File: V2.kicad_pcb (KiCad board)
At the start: 2 copper layers, 54.1 x 26 mm, 13 parts, among them SW1 SW_SPST, U1 CH32V003JxMx

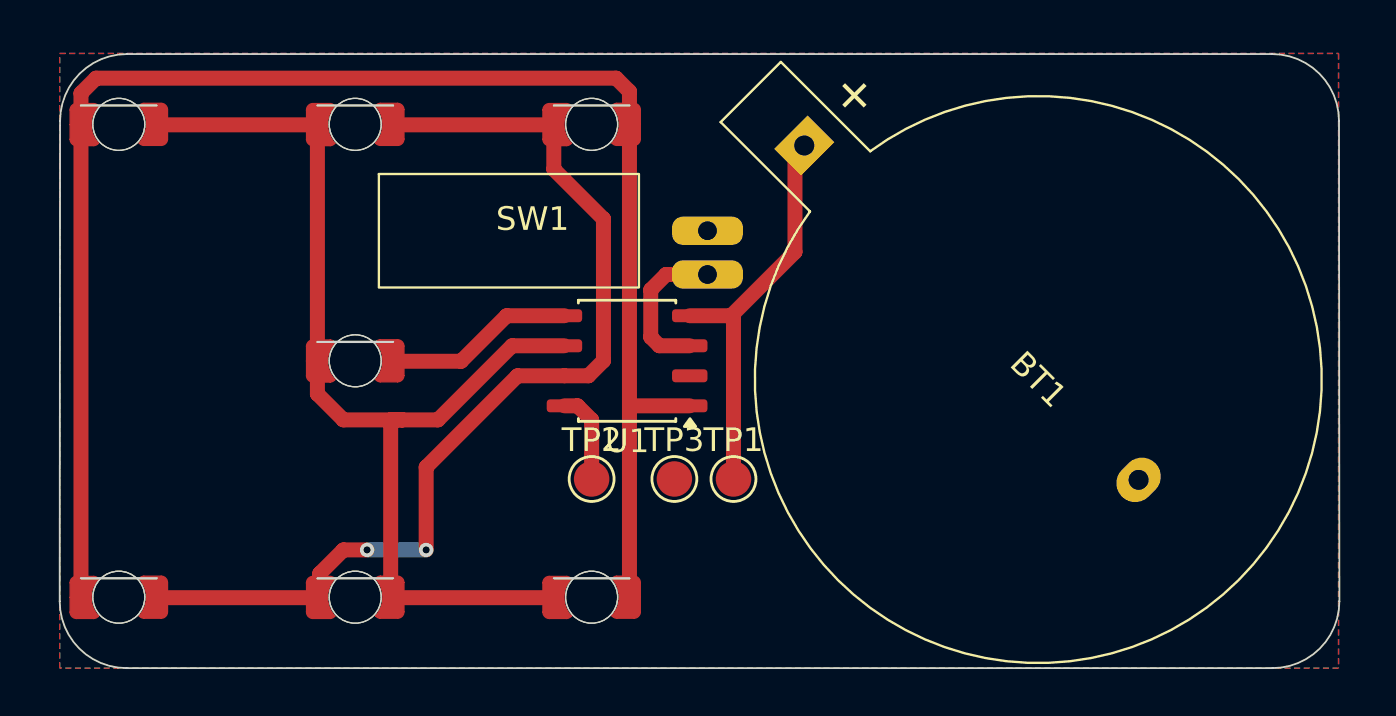
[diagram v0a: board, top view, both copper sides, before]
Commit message: final?
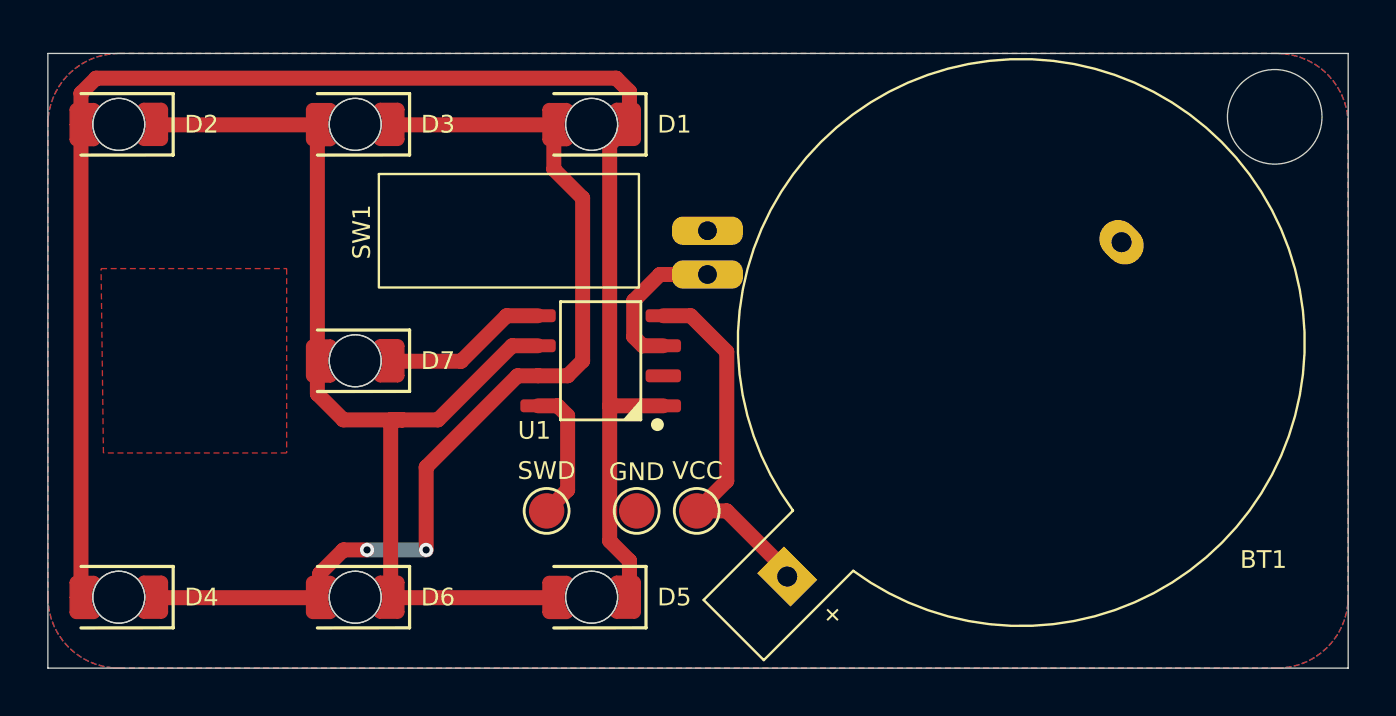
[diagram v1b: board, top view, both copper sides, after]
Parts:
- added REF**: MountingHole_4mm, MountingHole:MountingHole_4mm, F.Cu at (161.9, 69.6)
- moved SWD 2.33 mm to (131.1, 86.3)
- moved GND 2.09 mm to (134.9, 86.3)
- moved VCC 2.06 mm to (137.4, 86.3)
- moved BT1 1.72 mm to (151.1, 79.2), turned to 45 degrees
- moved U1 1.12 mm to (133.3, 80.0)
- renumbered TP3 to GND, TP2 to SWD, TP1 to VCC
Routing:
- net /PD1: track 3.90 -> 5.82 mm
- net +BATT: track 17.3 -> 15.7 mm
- net /PC4: track 43.3 -> 42.1 mm
- net /PC1: track 8.05 -> 6.93 mm
- net /PC2: track 45.3 -> 44.2 mm
- net /PA2: track 7.47 -> 6.52 mm
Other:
- board size 54.1 x 26 mm -> 55 x 26 mm
- board text added: "Detská univerzita 2026 TUKE"
- board text added: "kte.website.tuke.sk"
